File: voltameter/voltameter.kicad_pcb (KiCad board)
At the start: 2 copper layers, 16 parts, among them J1 Screw_Terminal_01x02, U1 4017, U2 NE555P

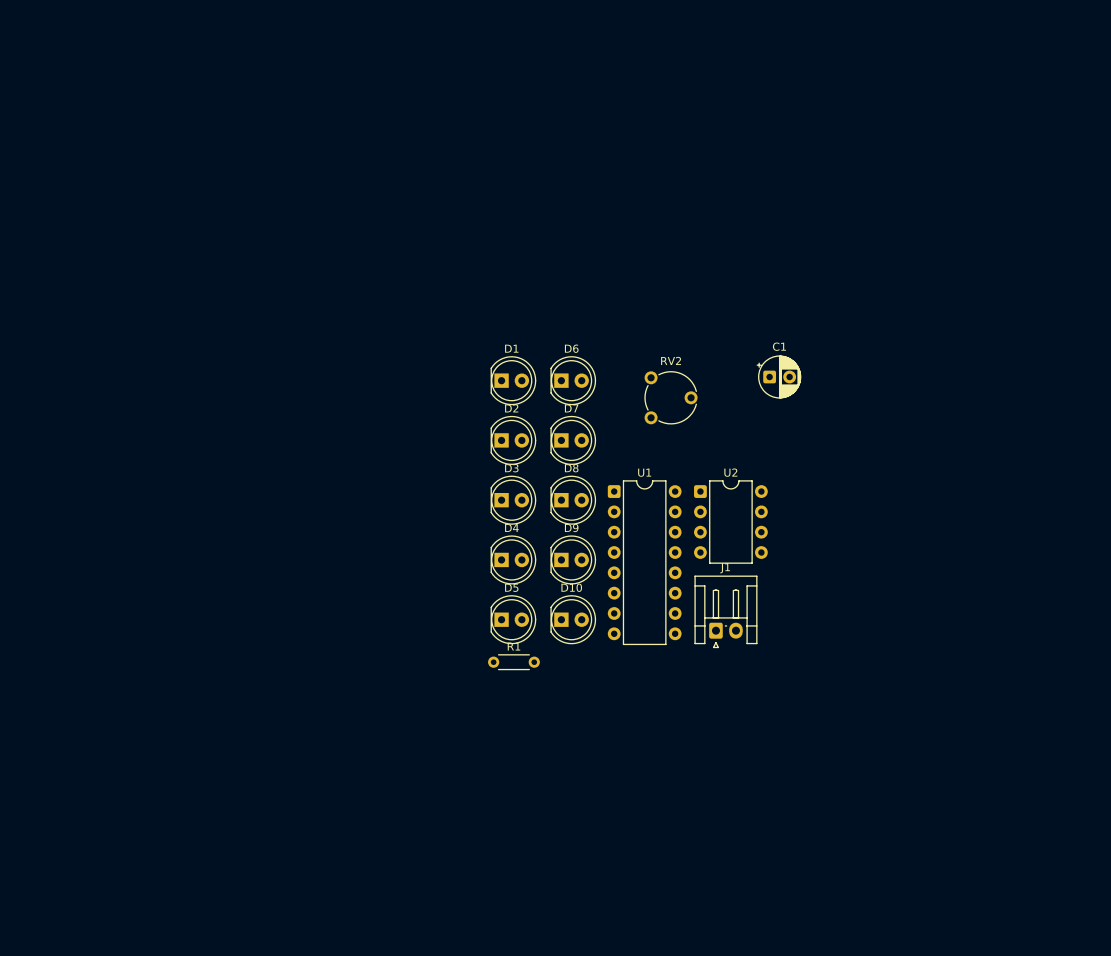
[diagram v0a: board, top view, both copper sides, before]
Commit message: refresh
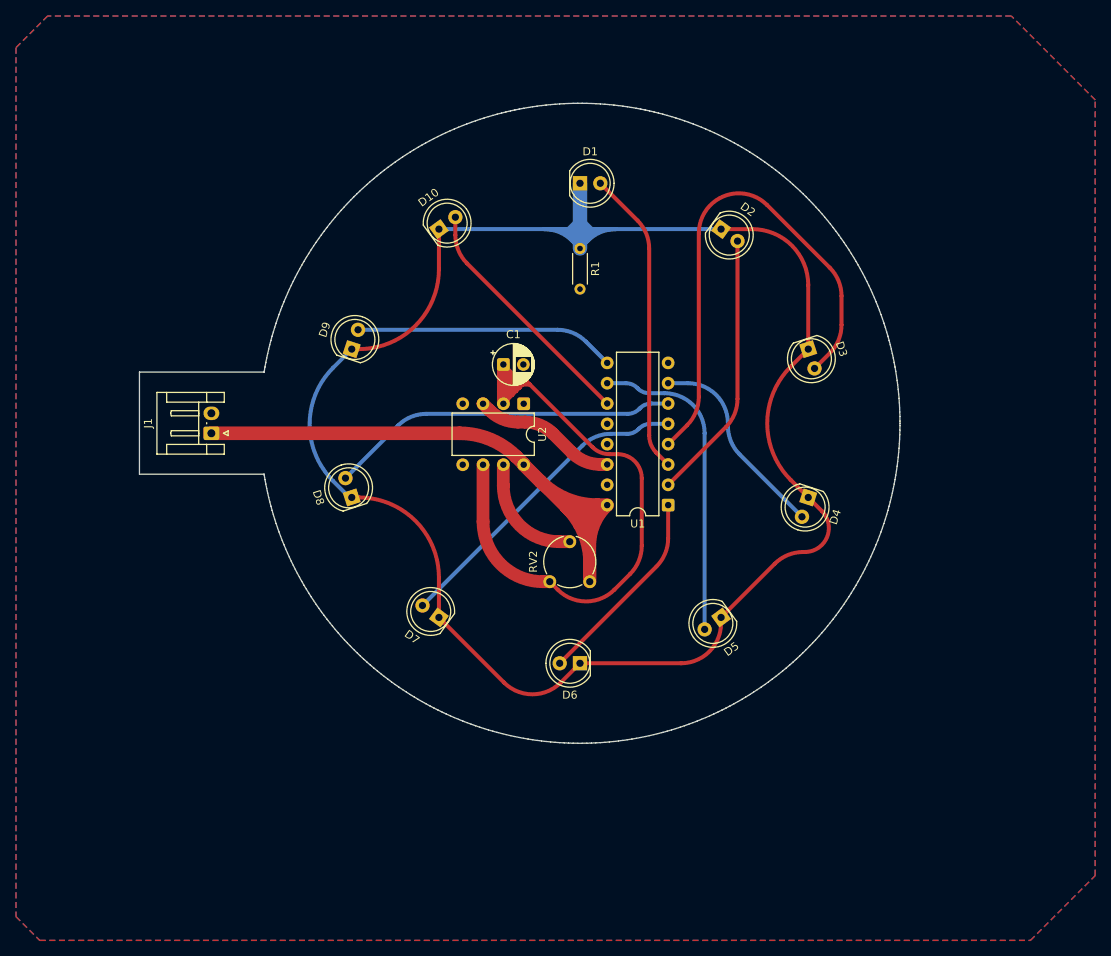
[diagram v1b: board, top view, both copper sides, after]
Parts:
- moved J1 67.7 mm to (126.5, 82.7), turned to 90 degrees
- moved R1 52.8 mm to (172.5, 59.5), turned to -90 degrees
- moved D10 51.2 mm to (154.9, 57.1), turned to 36 degrees
- moved D3 42.7 mm to (201.1, 72.1), turned to -72 degrees
- moved D4 39.1 mm to (201.1, 90.7), turned to -108 degrees
- moved D2 38.1 mm to (190.2, 57.1), turned to -36 degrees
- moved D9 37.2 mm to (144.0, 72.1), turned to 72 degrees
- moved D6 35.4 mm to (172.5, 111.4), turned to 180 degrees
- moved C1 33.3 mm to (162.9, 74.0)
- moved D5 27.4 mm to (190.2, 105.7), turned to -144 degrees
- moved D7 26.9 mm to (154.9, 105.7), turned to 144 degrees
- moved D1 26.6 mm to (172.5, 51.4)
- moved D8 26.2 mm to (144.0, 90.7), turned to 108 degrees
- moved U2 24.7 mm to (165.5, 79.0), turned to -90 degrees
- moved RV2 21.9 mm to (173.8, 101.2), turned to 90 degrees
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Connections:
- J1 pad 1: GND -> +9V
- J1 pad 2: +9V -> GND
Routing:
- net Net-(D1-K): track 0.00 -> 258.3 mm
- net Net-(U2-THRES): track 0.00 -> 95.4 mm
- net +9V: track 0.00 -> 89.8 mm
- net Net-(D3-A): track 0.00 -> 64.0 mm
- net Net-(D8-A): track 0.00 -> 43.8 mm
- net Net-(D7-A): track 0.00 -> 39.7 mm
- net Net-(D5-A): track 0.00 -> 39.7 mm
- net Net-(D1-A): track 0.00 -> 38.3 mm
- net Net-(D2-A): track 0.00 -> 33.8 mm
- net Net-(D9-A): track 0.00 -> 32.6 mm
- net Net-(D10-A): track 0.00 -> 30.9 mm
- net Net-(D4-A): track 0.00 -> 25.4 mm
- net Net-(D6-A): track 0.00 -> 25.1 mm
- net Net-(U1-CLK): track 0.00 -> 17.9 mm
- net Net-(U2-DISCH): track 0.00 -> 14.6 mm
- added copper zone on B.Cu, net GND
- added copper zone on F.Cu, net GND
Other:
- board outline added: 95.1 x 80 mm
- copper layers 2 -> 4
